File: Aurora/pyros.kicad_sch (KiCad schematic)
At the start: 16 parts, among them J10 Screw_Terminal_01x02, J11 Screw_Terminal_01x02, J12 Screw_Terminal_01x04, J13 Screw_Terminal_01x02, J14 Screw_Terminal_01x02, J15 Screw_Terminal_01x02, J17 Screw_Terminal_01x04, J18 Screw_Terminal_01x04, J2 Screw_Terminal_01x04, J22 Screw_Terminal_01x08, J23 Screw_Terminal_01x08, J24 Screw_Terminal_01x08, J25 Screw_Terminal_01x08, J7 Screw_Terminal_01x04, J8 Screw_Terminal_01x02, J9 Screw_Terminal_01x04

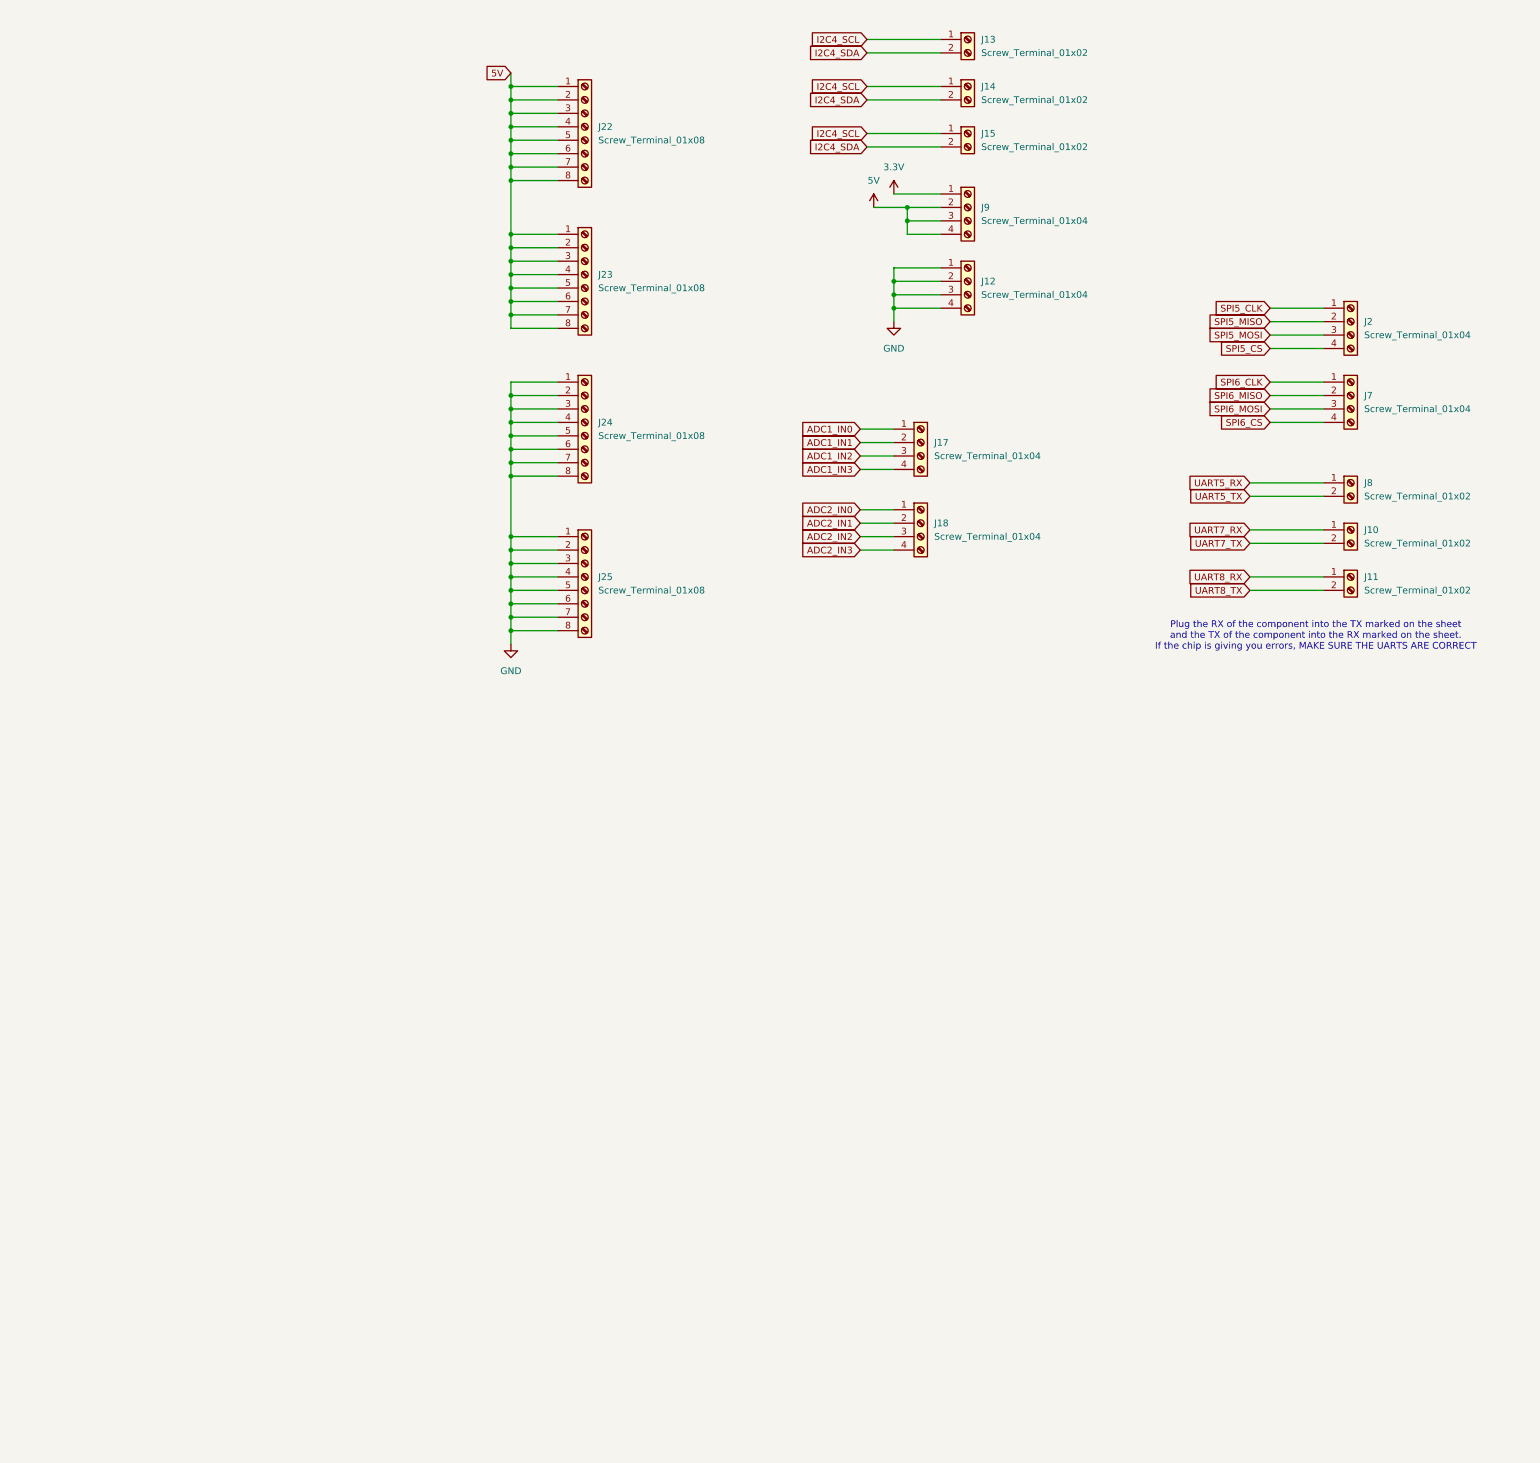
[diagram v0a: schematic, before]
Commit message: Add files via upload
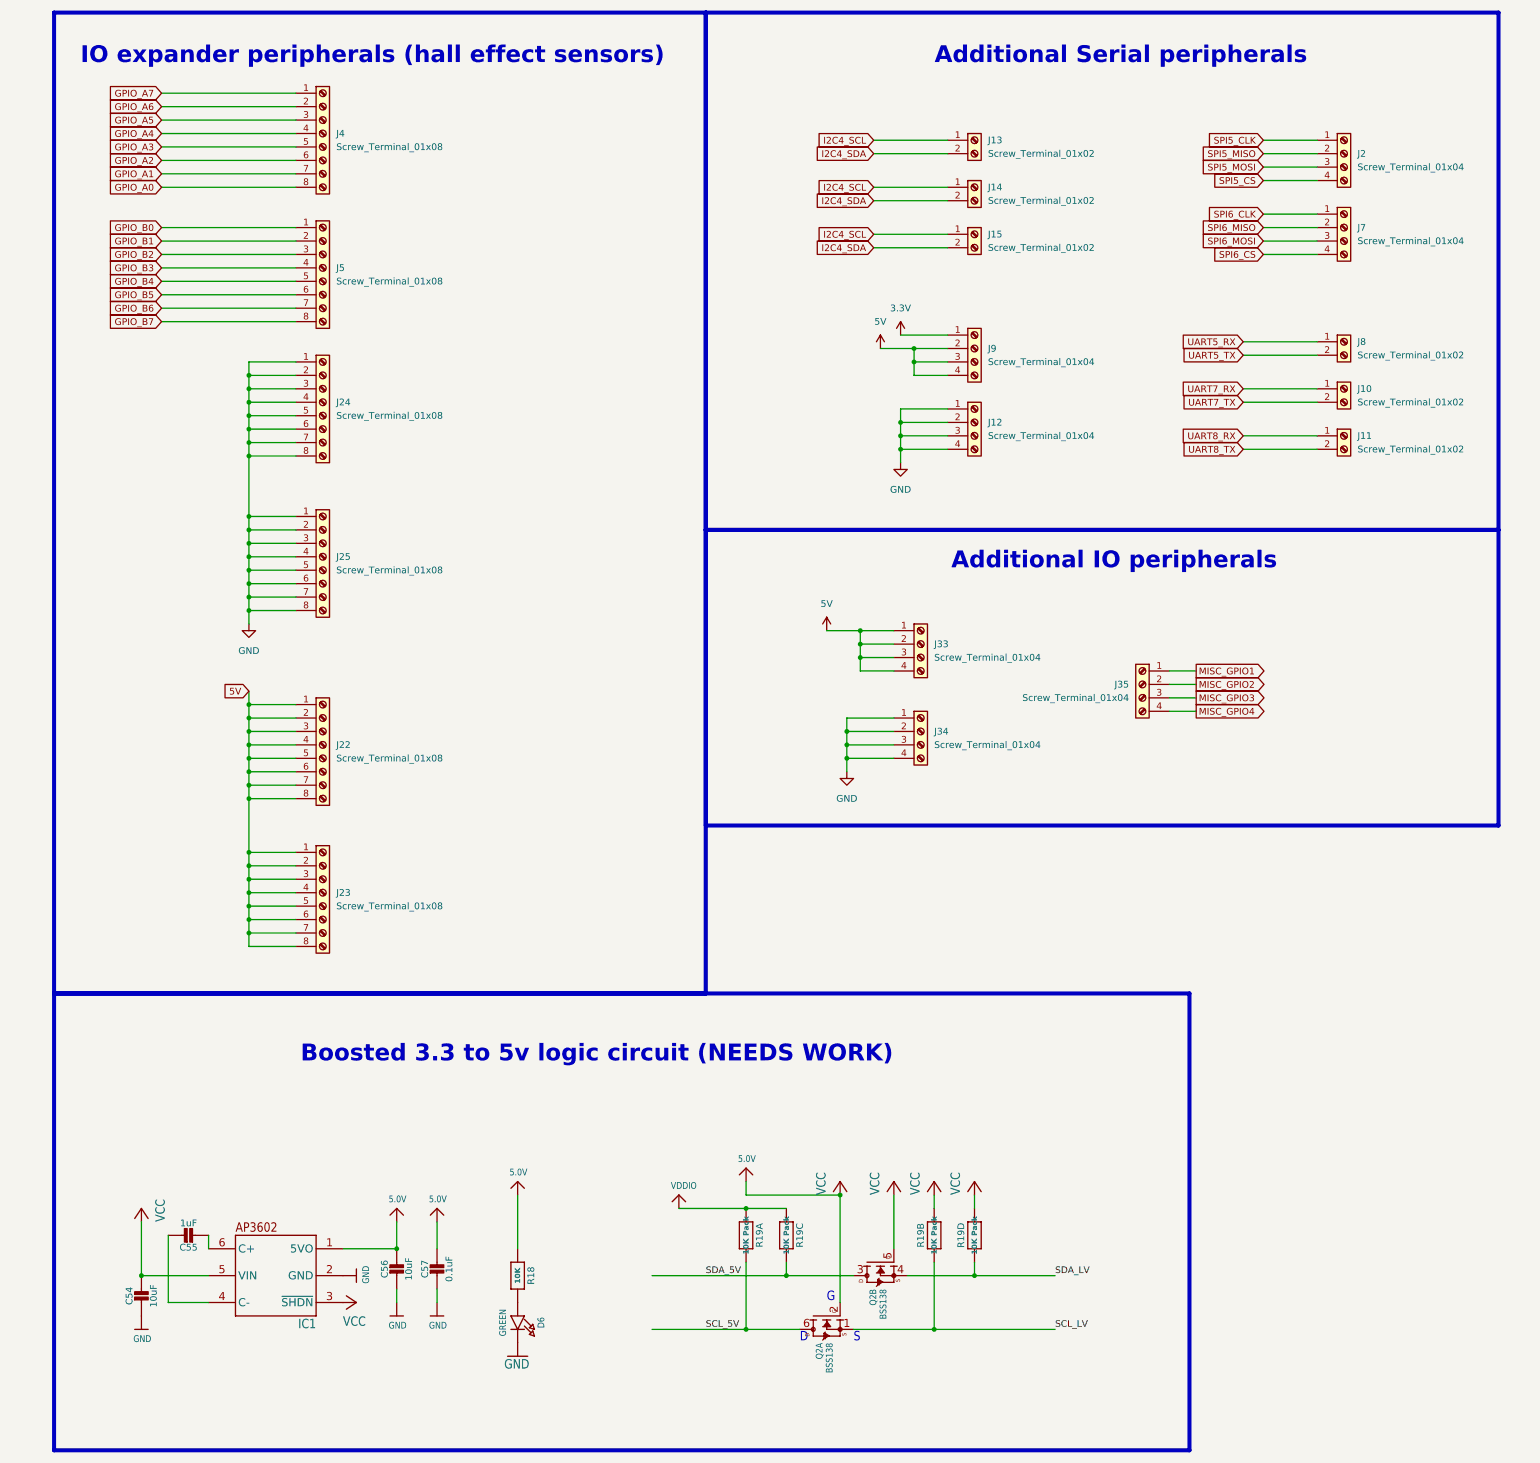
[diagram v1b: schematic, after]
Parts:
- removed J17, J18: Screw_Terminal_01x04, footprints6:CONN_1715747_PXC, symbol Connector:Screw_Terminal_01x04
- added C54, C56: 10uF, test:0805-NO, symbol test-eagle-import:CAP_CERAMIC0805-NOOUTLINE
- added C55: 1uF, test:0805-NO, symbol test-eagle-import:CAP_CERAMIC0805-NOOUTLINE
- added C57: 0.1uF, test:0603-NO, symbol test-eagle-import:CAP_CERAMIC0603_NO
- added D6: GREEN, test:CHIPLED_0603_NOOUTLINE, symbol test-eagle-import:LED0603_NOOUTLINE
- added IC1: AP3602/RT9361, test:SOT23-6, symbol test-eagle-import:AP3602
- added J33, J34, J35: Screw_Terminal_01x04, footprints6:CONN_1715747_PXC, symbol Connector:Screw_Terminal_01x04
- added J4, J5: Screw_Terminal_01x08, footprints7:CONN_1715789_PXC, symbol Connector:Screw_Terminal_01x08
- added Q2: BSS138, test:SOT363, symbol test-eagle-import:MOSFET-N_DUAL
- added R18: 10K, test:0603-NO, symbol test-eagle-import:RESISTOR_0603_NOOUT
- added R19: 10K Pack, test:RESPACK_4X0603, symbol test-eagle-import:RESISTOR_4PACK
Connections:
- net 5V: now also J33.1 (Pin_1), J33.2 (Pin_2), J33.3 (Pin_3), J33.4 (Pin_4)
- net GND: now also C54.2, C56.2, C57.2, D6.C, IC1.2 (GND), J34.1 (Pin_1), J34.2 (Pin_2), J34.3 (Pin_3), J34.4 (Pin_4)
- new net: D6.A, R18.2
- new net: C55.1, IC1.4 (C-)
- new net: C55.2, IC1.6 (C+)
- new net 5.0V: C54.1, C56.1, C57.1, IC1.1 (5VO), IC1.3 (~{SHDN}), IC1.5 (VIN), Q2.2 (G), Q2.5 (G), R18.1, R19.2 (1), R19.4 (1)
- new net GPIO_A0: J4.8 (Pin_8)
- new net GPIO_A1: J4.7 (Pin_7)
- new net GPIO_A2: J4.6 (Pin_6)
- new net GPIO_A3: J4.5 (Pin_5)
- new net GPIO_A4: J4.4 (Pin_4)
- new net GPIO_A5: J4.3 (Pin_3)
- new net GPIO_A6: J4.2 (Pin_2)
- new net GPIO_A7: J4.1 (Pin_1)
- new net GPIO_B0: J5.1 (Pin_1)
- new net GPIO_B1: J5.2 (Pin_2)
- new net GPIO_B2: J5.3 (Pin_3)
- new net GPIO_B3: J5.4 (Pin_4)
- new net GPIO_B4: J5.5 (Pin_5)
- new net GPIO_B5: J5.6 (Pin_6)
- new net GPIO_B6: J5.7 (Pin_7)
- new net GPIO_B7: J5.8 (Pin_8)
- new net MISC_GPIO1: J35.1 (Pin_1)
- new net MISC_GPIO2: J35.2 (Pin_2)
- new net MISC_GPIO3: J35.3 (Pin_3)
- new net MISC_GPIO4: J35.4 (Pin_4)
- new net SCL_5V: Q2.6 (D), R19.8 (2)
- new net SCL_LV: Q2.1 (S), R19.7 (2)
- new net SDA_5V: Q2.3 (D), R19.6 (2)
- new net SDA_LV: Q2.4 (S), R19.5 (2)
- new net VDDIO: R19.1, R19.3 (1)
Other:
- note added: "Additional IO peripherals"
- note added: "Additional Serial peripherals"
- note added: "Boosted 3.3 to 5v logic circuit (NEEDS WORK)"
- note added: "D"
- note added: "G"
- note added: "IO expander peripherals (hall effect sensors)"
- note added: "S"
- note removed: "Plug the RX of the component into the TX marked on the sheet and the TX of the component into the RX marked on the sheet. If the chip is giving you errors, MAKE SURE THE UARTS ARE CORRECT"
- moved on the sheet: J10, J11, J12, J13, J14, J15, J2, J22, J23, J24, J25, J7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
